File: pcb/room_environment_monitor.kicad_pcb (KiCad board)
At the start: 4 copper layers, 25.8 x 73 mm, 37 parts, among them J1 Conn_01x02_Pin, J2 Conn_01x04_Pin, J3 Conn_01x06_Socket, P1 USB_C_Plug_USB2.0, Q1 Q_Dual_NMOS_G1S2G2D2S1D1, Q3 BSS138, SW1 SW_SPST, U2 ESP32-C3-MINI-1, U3 SGP30-2.5K, U4 BME280, U5 AP2112K-3.3

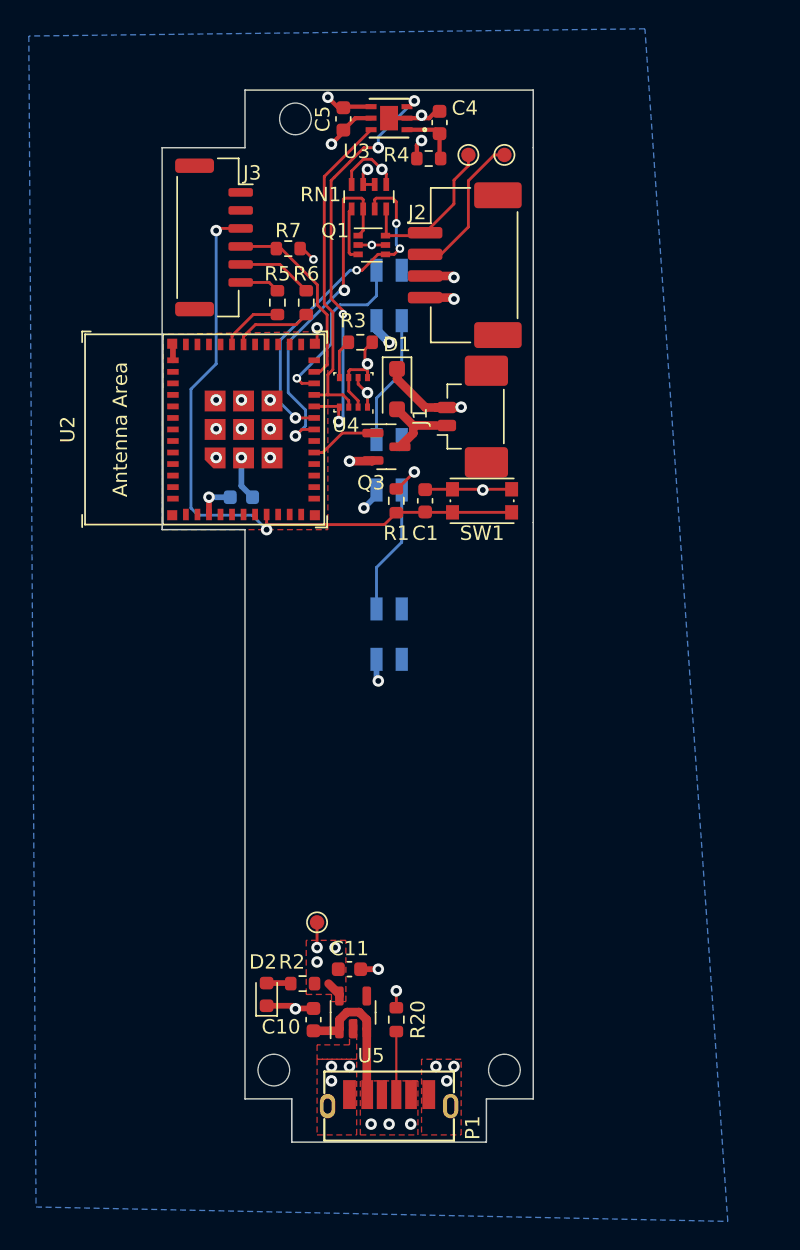
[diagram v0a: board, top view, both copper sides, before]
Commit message: finish routing the PCB
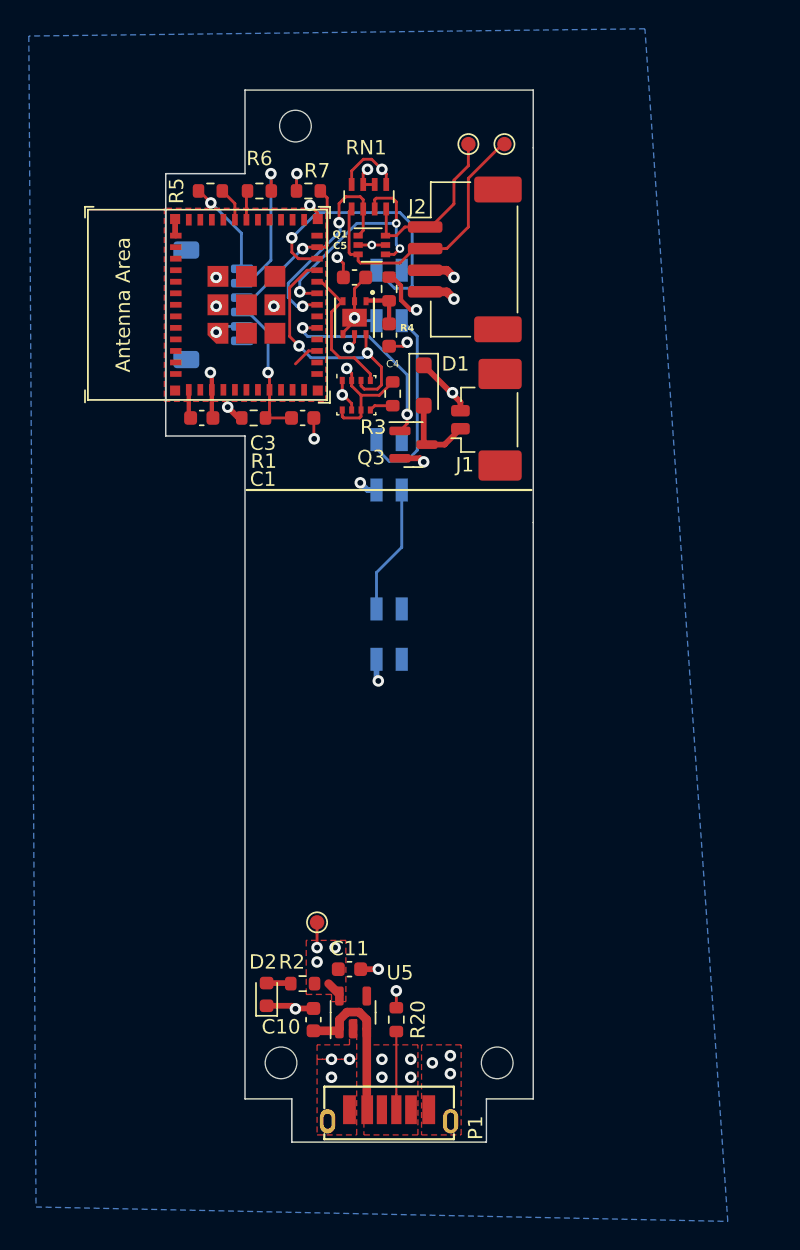
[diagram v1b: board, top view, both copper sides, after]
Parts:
- removed SW1: SW_SPST, Button_Switch_SMD:SW_Push_1P1T_NO_CK_KMR2
- C3: moved to F.Cu
- J3: footprint Connector_JST:JST_GH_SM06B-GHS-TB_1x06-1MP_P1.25mm_Horizontal -> Connector_JST:JST_SH_SM06B-SRSS-TB_1x06-1MP_P1.00mm_Horizontal; moved to B.Cu
- U3: footprint Kevin_Lutzer_Lbr:SGP30-2.5K_SEN-M -> Kevin_Lutzer_Lbr:SGP30-2.5K_SEN-L
- moved C4 15.2 mm to (110.0, 87.0), turned to -90 degrees
- moved U3 14.0 mm to (107.6, 85.8), turned to -90 degrees
- moved R1 11.4 mm to (100.6, 92.8), turned to 0 degrees
- moved C5 11.0 mm to (107.6, 83.0), turned to 0 degrees
- moved C1 10.3 mm to (104.0, 92.8), turned to 0 degrees
- moved R4 9.46 mm to (110.0, 83.8), turned to -90 degrees
- moved R5 9.04 mm to (97.6, 77.0), turned to 180 degrees
- moved U2 8.65 mm to (97.4, 84.9)
- moved R6 8.40 mm to (101.0, 77.0), turned to 0 degrees
- moved C3 6.15 mm to (97.0, 92.8), turned to 180 degrees
- moved J3 4.68 mm to (97.8, 84.9), turned to 90 degrees
- moved R7 4.24 mm to (104.4, 77.0), turned to 0 degrees
- moved R3 4.22 mm to (110.2, 91.1), turned to -90 degrees
- moved Q3 1.88 mm to (111.7, 94.6)
- moved D1 1.87 mm to (112.4, 90.5)
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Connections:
- J1 pad 1: +5V -> Net-(D1-A)
- J1 pad 2: Net-(D1-A) -> +5V
- J3 pad 1: unconnected-(J3-Pin_1-Pad1) -> +5V
- J3 pad 2: unconnected-(J3-Pin_2-Pad2) -> GND
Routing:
- net EN: track 45.6 -> 9.90 mm, vias 2 -> 1
- net I2C_SCL: track 29.2 -> 9.62 mm, vias 4 -> 0
- net UART1_RX_LVL: track 24.7 -> 15.0 mm
- net FAN: track 4.63 -> 13.8 mm, vias 0 -> 2
- net NEOPIXEL: track 12.2 -> 19.7 mm
- net UART1_TX_LVL: track 23.7 -> 17.2 mm, vias 4 -> 3
- net UART1_TX: track 14.0 -> 19.8 mm
- net I2C_SDA: track 23.2 -> 17.9 mm, vias 0 -> 2
- net Net-(J3-Pin_5): track 5.31 -> 9.88 mm, vias 0 -> 1
- net Net-(D3-DOUT): track 8.97 -> 12.9 mm
- net Net-(J3-Pin_6): track 2.79 -> 6.66 mm, vias 0 -> 1
- net UART_RX: track 5.53 -> 1.92 mm
- net GND: track 35.2 -> 31.9 mm, vias 28 -> 22
- net +3V3: track 22.1 -> 24.9 mm, vias 10 -> 11
- net UART_TX: track 4.36 -> 2.36 mm
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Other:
- board size 25.8 x 73 mm -> 25.5 x 73 mm

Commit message: finish v4 and the images for doucmentation
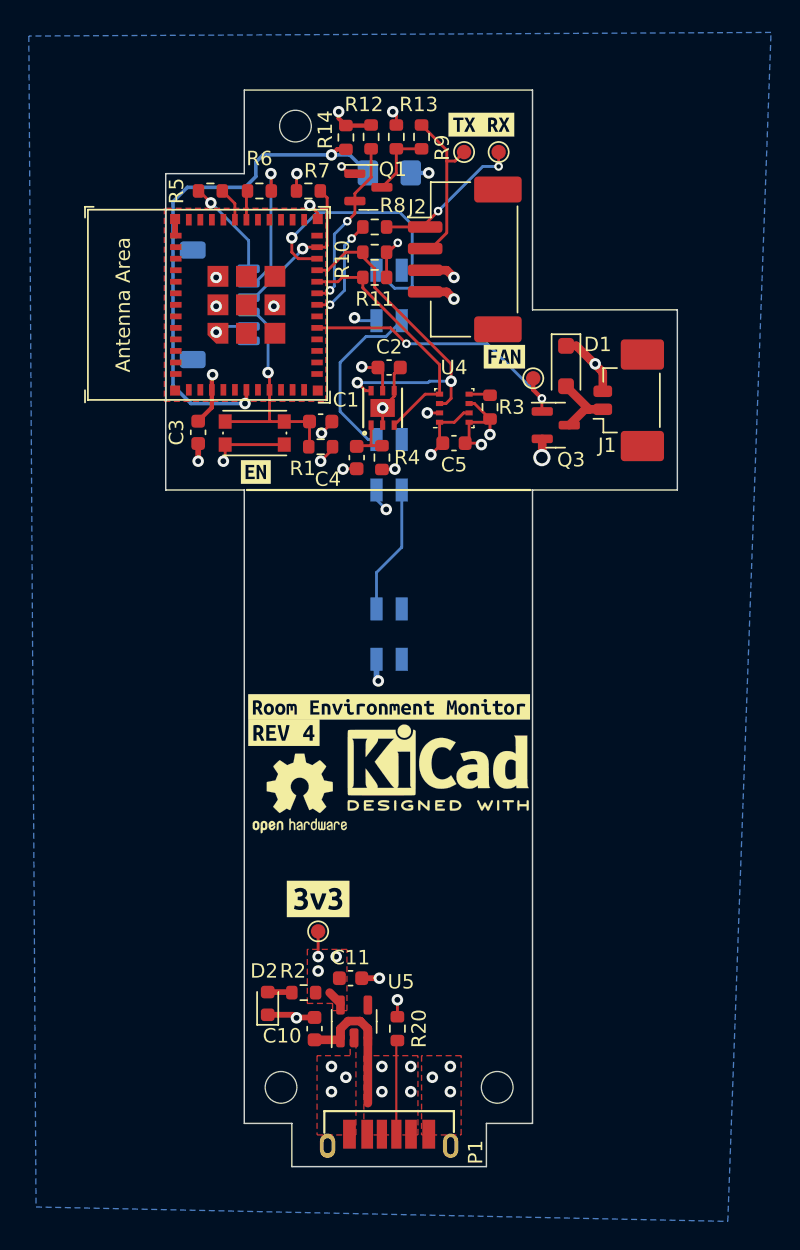
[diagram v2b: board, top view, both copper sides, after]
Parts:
- removed RN1: 10k, Resistor_SMD:R_Array_Concave_4x0603
- added C2: 0u1, Capacitor_SMD:C_0603_1608Metric, F.Cu at (110.0, 89.2)
- added D6: D_Photo, Diode_SMD:D_1206_3216Metric_Pad1.42x1.75mm_HandSolder, B.Cu at (110.0, 75.8)
- added R10: 2k2, Resistor_SMD:R_0603_1608Metric, F.Cu at (109.0, 81.2)
- added R11: 2k2, Resistor_SMD:R_0603_1608Metric, F.Cu at (109.0, 83.0)
- added R12: 10k, Resistor_SMD:R_0603_1608Metric, F.Cu at (108.8, 73.2)
- added R13: 10k, Resistor_SMD:R_0603_1608Metric, F.Cu at (110.5, 73.2)
- added R14: R_Small_US, Resistor_SMD:R_0603_1608Metric, F.Cu at (107.0, 73.3)
- added R8: 0, Resistor_SMD:R_0603_1608Metric, F.Cu at (109.0, 79.5)
- added R9: 0, Resistor_SMD:R_0603_1608Metric, F.Cu at (112.2, 73.2)
- added REF**: KiCad-Logo2_5mm_SilkScreen, Symbol:KiCad-Logo2_5mm_SilkScreen, F.Cu at (113.4, 117.0)
- added REF**: OSHW-Logo2_7.3x6mm_SilkScreen, Symbol:OSHW-Logo2_7.3x6mm_SilkScreen, F.Cu at (103.8, 118.8)
- added SW1: SW_SPST, Button_Switch_SMD:SW_Push_1P1T_NO_CK_KMR2, F.Cu at (100.7, 93.8)
- added TP1: TestPoint, TestPoint:TestPoint_Pad_D1.0mm, F.Cu at (120.0, 90.0)
- added kibuzzard-652F08CD: G***, kibuzzard-652F08CD, F.Cu at (116.4, 72.4)
- added kibuzzard-652F0EDE: G***, kibuzzard-652F0EDE, F.Cu at (105.1, 126.1)
- added kibuzzard-652F0FC5: G***, kibuzzard-652F0FC5, F.Cu at (118.0, 88.5)
- added kibuzzard-652F2D51: G***, kibuzzard-652F2D51, F.Cu at (100.8, 96.5)
- added kibuzzard-652F50CA: G***, kibuzzard-652F50CA, F.Cu at (110.0, 112.8)
- added kibuzzard-652F5449: G***, kibuzzard-652F5449, F.Cu at (102.7, 114.6)
- C1, C4, C5: value 100n -> 0u1
- C3: value 0.1u -> 0u1
- D1: value MBR1020VL -> CDBMS160
- Q1: value Q_Dual_NMOS_G1S2G2D2S1D1 -> BSS138; footprint Package_TO_SOT_SMD:SOT-363_SC-70-6 -> Package_TO_SOT_SMD:SOT-23
- U3: footprint Kevin_Lutzer_Lbr:SGP30-2.5K_SEN-L -> Kevin_Lutzer_Lbr:SGP30-2.5K_SEN
- moved C5 13.4 mm to (114.5, 94.5), turned to 180 degrees
- moved R4 11.7 mm to (109.5, 95.5), turned to 90 degrees
- moved D1 9.97 mm to (122.3, 89.2)
- moved J1 9.97 mm to (126.1, 91.5)
- moved Q3 9.97 mm to (121.6, 93.2)
- moved C4 8.79 mm to (107.8, 95.5)
- moved U4 6.86 mm to (114.5, 92.1), turned to 90 degrees
- moved R3 6.81 mm to (117.0, 92.0), turned to 90 degrees
- moved U3 6.56 mm to (109.6, 92.1), turned to 90 degrees
- moved R1 5.06 mm to (105.2, 94.8), turned to 180 degrees
- moved Q1 4.01 mm to (108.6, 76.8)
- moved TP3 2.85 mm to (115.2, 74.3)
- moved TP2 2.17 mm to (117.6, 74.3)
- moved H1 1.70 mm to (102.5, 139.2)
- moved H2 1.70 mm to (117.5, 139.2)
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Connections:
- J2 pad 1: UART1_RX -> Net-(J2-Pin_1)
- J2 pad 2: UART1_TX -> Net-(J2-Pin_2)
- Q1 pad 1: UART1_RX_LVL -> +3V3
- Q1 pad 2: +5V -> UART1_TX_LVL
- TP2 pad 1: UART1_RX -> Net-(J2-Pin_1)
- TP3 pad 1: UART1_TX -> Net-(J2-Pin_2)
- U2 pad 18: UART1_RX_LVL -> UART1_RX
- U2 pad 6: unconnected-(U2-GPIO3/ADC1_CH3-Pad6) -> PD
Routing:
- net PD: track 0.00 -> 36.4 mm, vias 0 -> 2
- net UART1_TX: track 19.8 -> 4.84 mm
- net UART1_RX_LVL: track 15.0 -> 0.00 mm, vias 2 -> 0
- net Net-(J2-Pin_2): track 0.00 -> 11.1 mm
- net Net-(J2-Pin_1): track 0.00 -> 10.4 mm, vias 0 -> 2
- net I2C_SCL: track 9.62 -> 17.6 mm
- net I2C_SDA: track 17.9 -> 24.7 mm
- net FAN: track 13.8 -> 20.2 mm
- net EN: track 9.90 -> 15.6 mm
- net +5V: track 23.2 -> 17.9 mm, vias 8 -> 7
- net GND: track 31.9 -> 37.1 mm, vias 22 -> 26
- net UART1_TX_LVL: track 17.2 -> 12.0 mm, vias 3 -> 2
- net UART1_RX: track 12.0 -> 7.22 mm, vias 0 -> 2
- net /Sensors/SGP30_VDD: track 4.79 -> 3.15 mm
- net +3V3: track 24.9 -> 26.3 mm, vias 11 -> 14
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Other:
- board size 25.5 x 73 mm -> 35.5 x 74.7 mm
